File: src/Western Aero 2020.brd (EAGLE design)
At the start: 127.7 x 105.9 mm, 94 parts, among them IC1 LT1963AET, IC2 LT1963AET, J1 PITOT, J10 ANA_IO, J11 PWR, J12 POWER, J2 BUZZER, J3 RX2/TX2, J4 RX3/TX3, J5 SPI, J6 DIG_IO, J7 RX1/TX1, J8 DIG_IO, J9 REF/GND, U3 TEENSY_3.5_DIL+4, U5 SPARKFUN_MPU9250_IMU, U6 ADAFRUIT_MPL3115A2_BAROMETER, U7 ADAFRUIT_INA219_BATTERY_SENSOR, U8 ADAFRUIT_RFM95W_LORA_RADIO, U9 ADAFRUIT_MTK3339_GPS

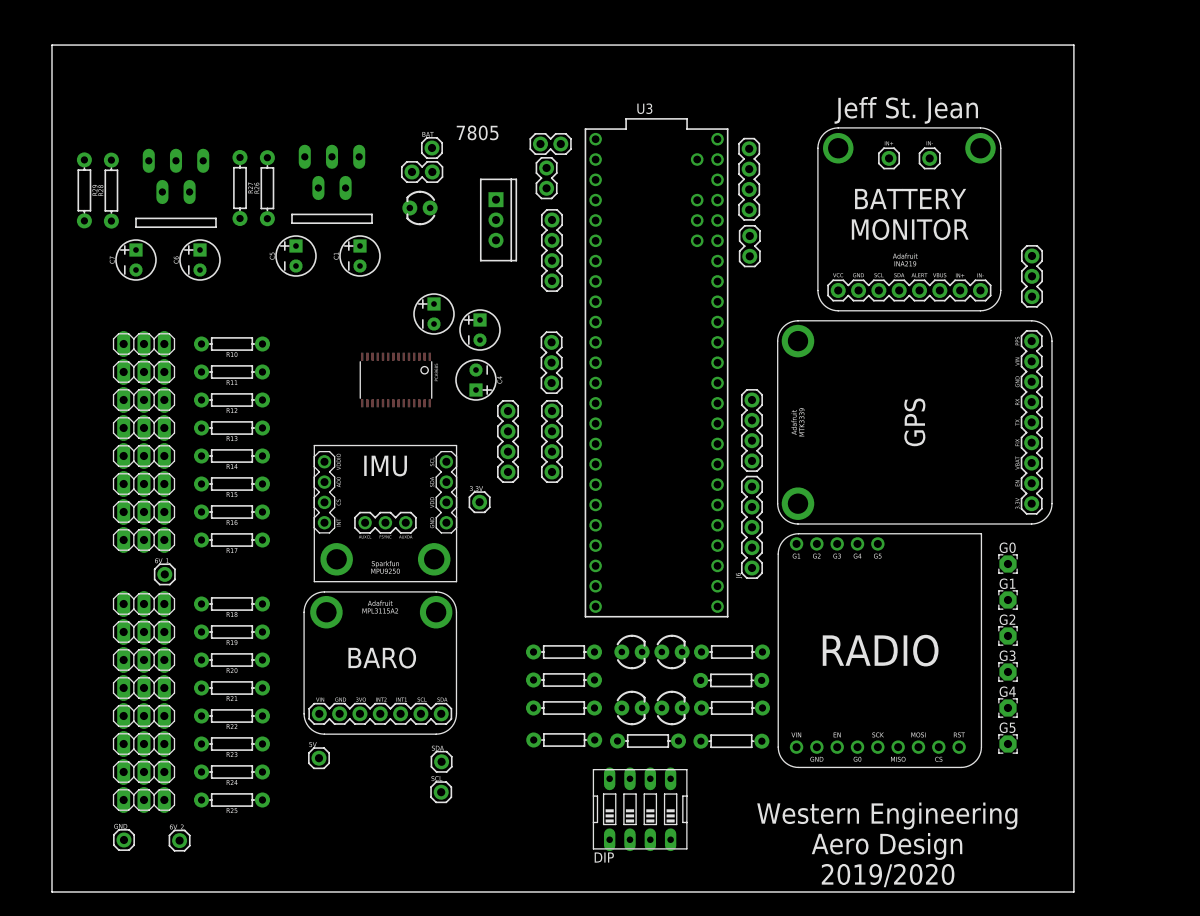
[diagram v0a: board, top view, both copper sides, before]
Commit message: Finished new route.
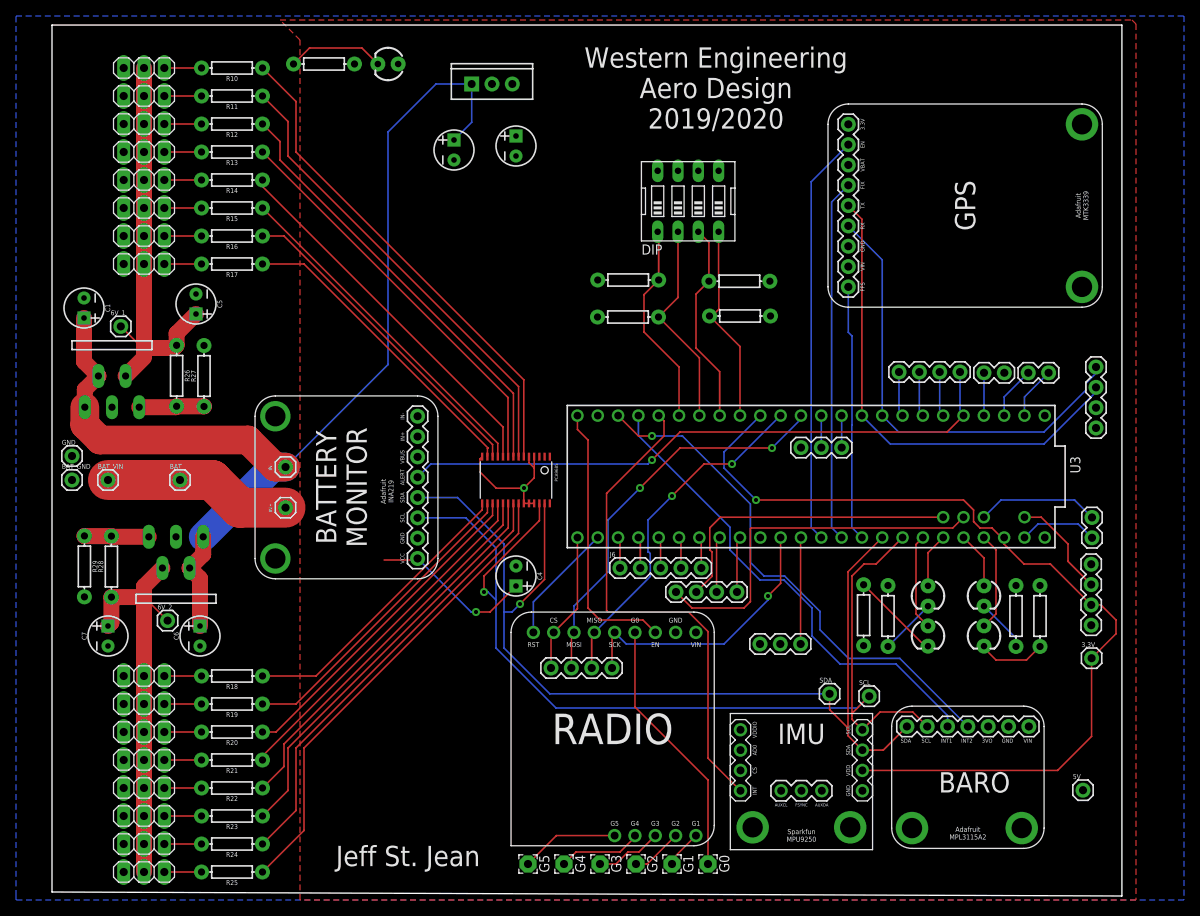
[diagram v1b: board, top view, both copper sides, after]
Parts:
- removed J12: POWER, SparkFun-Connectors:1X02
- added BAT_GND, BAT_VIN: (no value), SparkFun-Connectors:1X01
- moved 5V 95.6 mm to (127.4, 13.2)
- moved U6 92.6 mm to (122.5, 23.7), turned to 180 degrees
- moved R4 82.6 mm to (32.5, 104.0), turned to 180 degrees
- moved 3.3V 78.9 mm to (128.4, 29.7)
- moved DIP 76.2 mm to (78.0, 86.8)
- moved J4 73.7 mm to (129.0, 58.5)
- moved J11 73.3 mm to (128.4, 33.9), turned to 90 degrees
- moved J7 67.8 mm to (123.1, 65.4), turned to 180 degrees
- moved U5 61.9 mm to (83.3, 22.8)
- moved G5 61.8 mm to (58.0, 4.00), turned to 270 degrees
- moved J2 60.1 mm to (115.0, 65.4), turned to 0 degrees
- moved U9 59.5 mm to (95.5, 99.0), turned to 270 degrees
- moved J1 59.2 mm to (87.0, 31.5), turned to 0 degrees
- moved G4 58.8 mm to (62.5, 4.00), turned to 270 degrees
- moved U7 58.1 mm to (46.7, 39.6), turned to 90 degrees
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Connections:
- net GND: now also BAT_GND.1; no longer J12.1
- net VIN+: now also BAT_VIN.1; no longer J12.2
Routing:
- net VIN-: track 0.00 -> 136.4 mm
- net SCL: track 0.00 -> 131.0 mm, vias 0 -> 1
- net SDA: track 0.00 -> 126.7 mm, vias 0 -> 1
- net 3.3V: track 0.00 -> 112.9 mm, vias 0 -> 1
- net D3: track 0.00 -> 77.1 mm, vias 0 -> 1
- net ENV_INT2: track 0.00 -> 65.4 mm, vias 0 -> 1
- net IMU_INT: track 0.00 -> 63.0 mm
- net PWM0: track 0.00 -> 62.1 mm
- net TX3: track 0.00 -> 61.0 mm
- net ENV_INT1: track 0.00 -> 60.7 mm
- net PWM15: track 0.00 -> 59.3 mm
- net PWM1: track 0.00 -> 58.3 mm
- net RX3: track 0.00 -> 57.3 mm
- net PWM14: track 0.00 -> 55.6 mm
- net PWM2: track 0.00 -> 54.6 mm
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- added copper zone on layer 1, net 5V
- added copper zone on layer 16, net GND
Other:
- board size 127.7 x 105.9 mm -> 133.7 x 108.9 mm
- board text removed: "7805"
